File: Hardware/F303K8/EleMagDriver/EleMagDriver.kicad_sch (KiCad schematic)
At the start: 43 parts, among them IC1 BD9E302EFJ-E2, IC2 TBD62083APG, IC3 TBD62083APG, IC4 TBD62083APG, J1 Jack-DC, J10 RelayD, J11 RelayE, J12 RelayF, J13 RelayG, J14 RelayH, J15 RelayI, J16 RelayJ, J17 Floppy_Power, J18 FloppyA, J19 Floppy_Power, J2 MotorDriverIn, J20 FloppyB, J21 Floppy_Power, J22 FloppyC, J3 MotorDriveOut, J4 SolenoidA, J5 SolenoidB, J6 StpMotor, J7 RelayA, J8 RelayB, J9 RelayC, U1 NUCLEO-F303K8

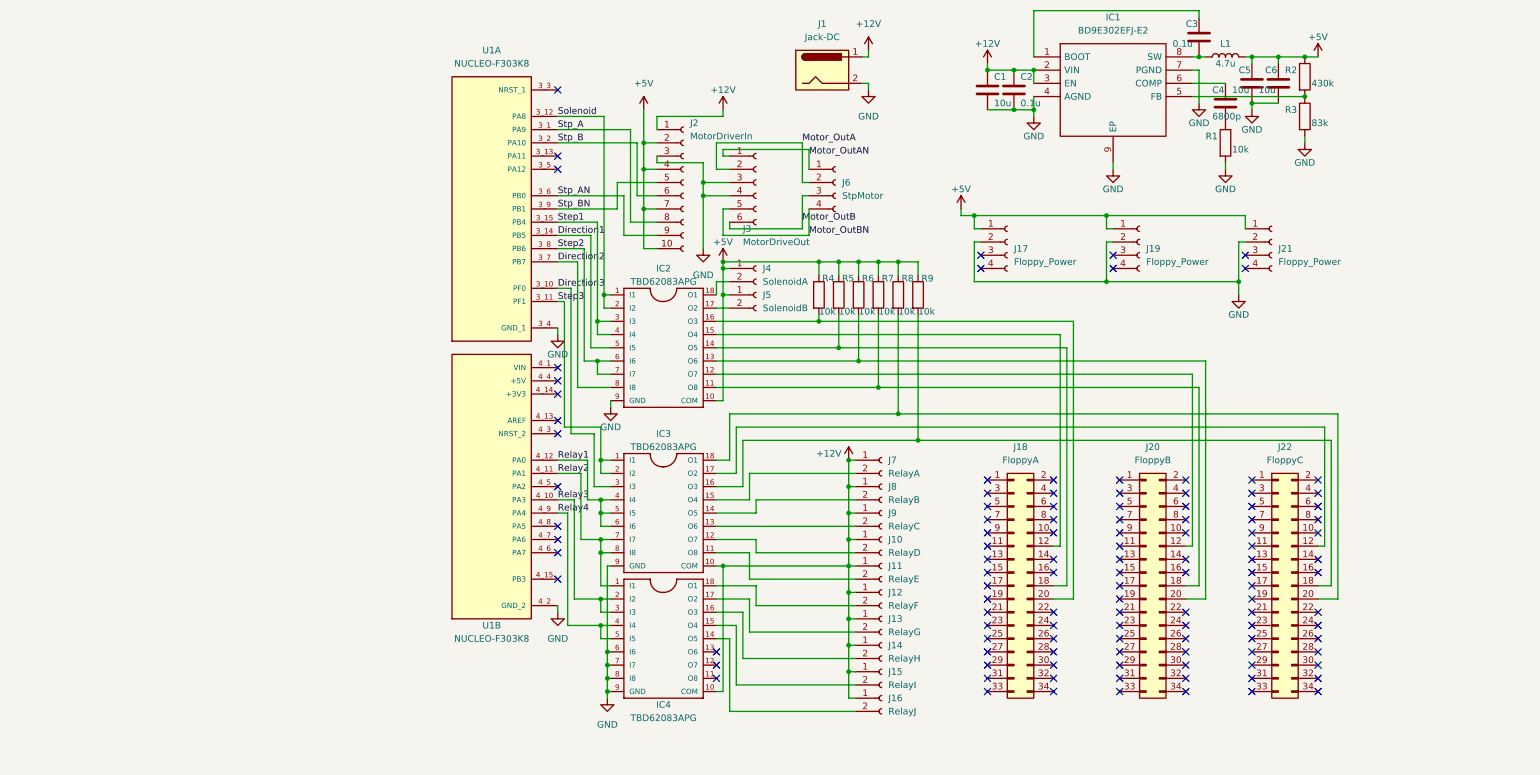
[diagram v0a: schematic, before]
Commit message: add SoundLevelMater
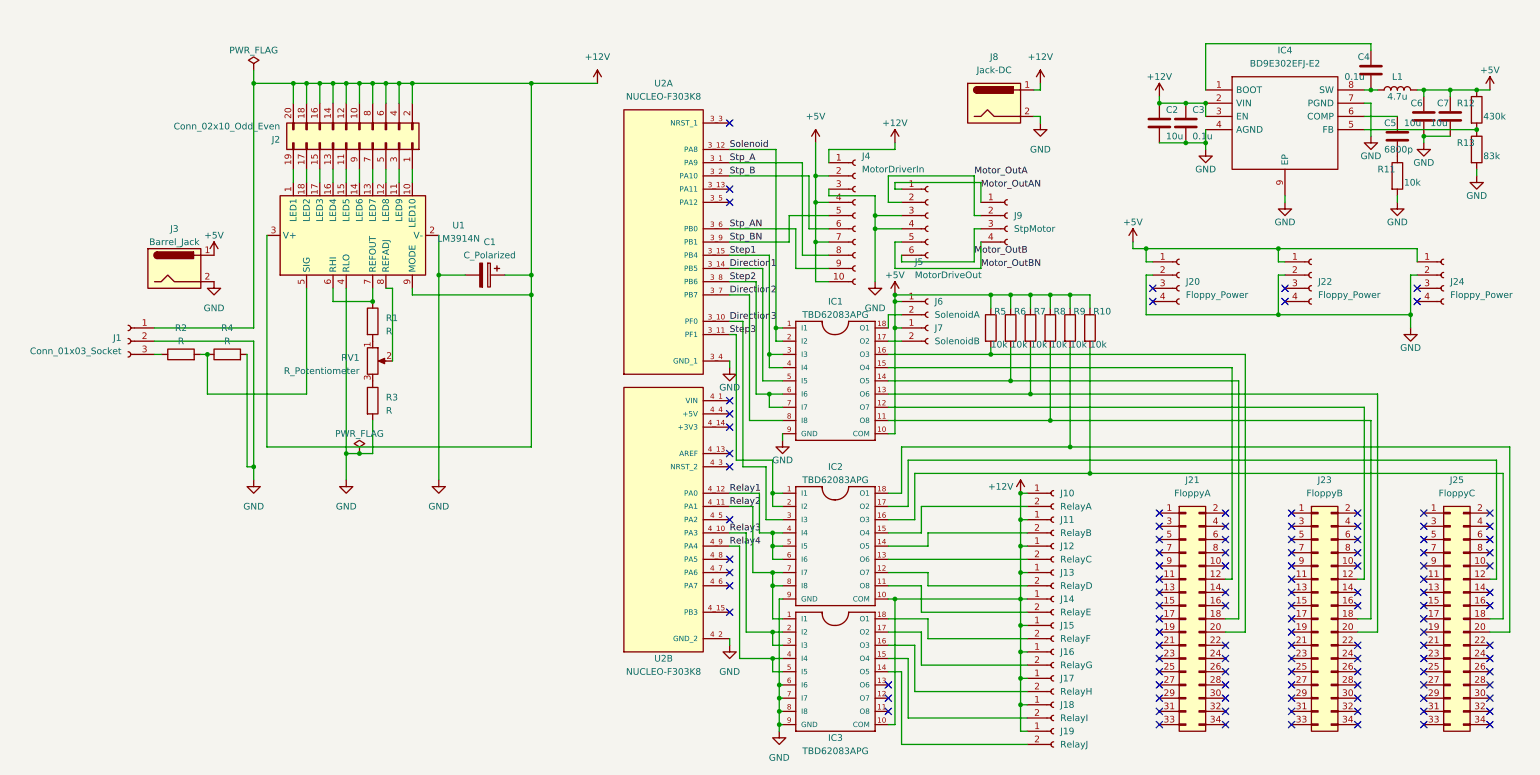
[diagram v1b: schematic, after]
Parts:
- added C1: C_Polarized, Capacitor_THT:CP_Radial_D5.0mm_P2.00mm, symbol Device:C_Polarized
- added J1: Conn_01x03_Socket, Connector_PinSocket_1.00mm:PinSocket_1x03_P1.00mm_Vertical, symbol Connector:Conn_01x03_Socket
- added J2: Conn_02x10_Odd_Even, Connector_PinSocket_2.00mm:PinSocket_2x10_P2.00mm_Vertical, symbol Connector_Generic:Conn_02x10_Odd_Even
- added J3: Barrel_Jack, Connector_BarrelJack:BarrelJack_SwitchcraftConxall_RAPC10U_Horizontal, symbol Connector:Barrel_Jack
- added R1, R2, R3, R4: R, Resistor_SMD:R_0402_1005Metric, symbol Device:R
- added RV1: R_Potentiometer, Potentiometer_THT:Potentiometer_ACP_CA6-H2,5_Horizontal, symbol Device:R_Potentiometer
- added U1: LM3914N, Package_DIP:DIP-18_W7.62mm, symbol Driver_LED:LM3914N
- renumbered C1 to C2, C2 to C3, C3 to C4, C4 to C5, C5 to C6, C6 to C7, IC2 to IC1, IC3 to IC2, IC4 to IC3, IC1 to IC4, J7 to J10, J8 to J11, J9 to J12, J10 to J13, J11 to J14, J12 to J15, J13 to J16, J14 to J17, J15 to J18, J16 to J19, J17 to J20, J18 to J21, J19 to J22, J20 to J23, J21 to J24, J22 to J25, J2 to J4, J3 to J5, J4 to J6, J5 to J7, J1 to J8, J6 to J9, R9 to R10, R1 to R11, R2 to R12, R3 to R13, R4 to R5, R5 to R6, R6 to R7, R7 to R8, R8 to R9, U1 to U2
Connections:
- net +12V: now also C1.1, J1.1 (Pin_1), J2.10 (Pin_10), J2.12 (Pin_12), J2.14 (Pin_14), J2.16 (Pin_16), J2.18 (Pin_18), J2.2 (Pin_2), J2.20 (Pin_20), J2.4 (Pin_4), J2.6 (Pin_6), J2.8 (Pin_8), U1.3 (V+), U1.9 (MODE)
- net +5V: now also J3.1
- net GND: now also C1.2, J1.2 (Pin_2), J3.2, R3.2, R4.2, U1.2 (V-), U1.4 (RLO)
- new net: J1.3 (Pin_3), R2.1
- new net: R1.2, RV1.1
- new net: RV1.2, U1.8 (REFADJ)
- new net: R3.1, RV1.3
- new net: J2.19 (Pin_19), U1.1 (LED1)
- new net: J2.1 (Pin_1), U1.10 (LED10)
- new net: J2.3 (Pin_3), U1.11 (LED9)
- new net: J2.5 (Pin_5), U1.12 (LED8)
- new net: J2.7 (Pin_7), U1.13 (LED7)
- new net: J2.9 (Pin_9), U1.14 (LED6)
- new net: J2.11 (Pin_11), U1.15 (LED5)
- new net: J2.13 (Pin_13), U1.16 (LED4)
- new net: J2.15 (Pin_15), U1.17 (LED3)
- new net: J2.17 (Pin_17), U1.18 (LED2)
- new net: R2.2, R4.1, U1.5 (SIG)
- new net: R1.1, U1.6 (RHI), U1.7 (REFOUT)
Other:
- moved on the sheet: C2, C3, C4, C5, C6, C7, IC1, IC2, IC3, IC4, J10, J11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
